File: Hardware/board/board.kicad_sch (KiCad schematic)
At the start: 0 parts

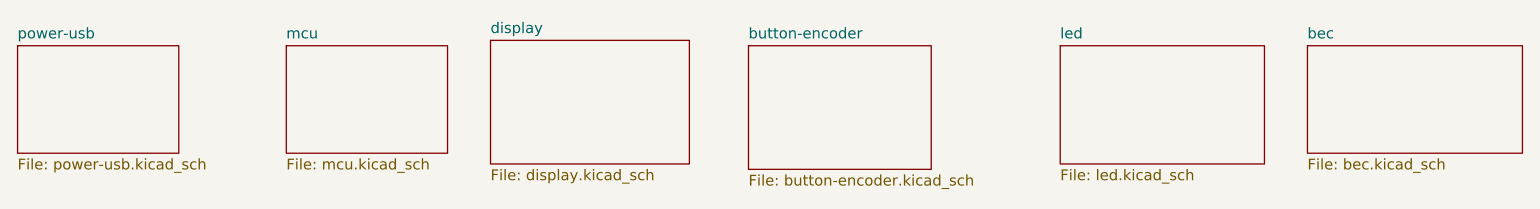
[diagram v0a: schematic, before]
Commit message: sdadsa
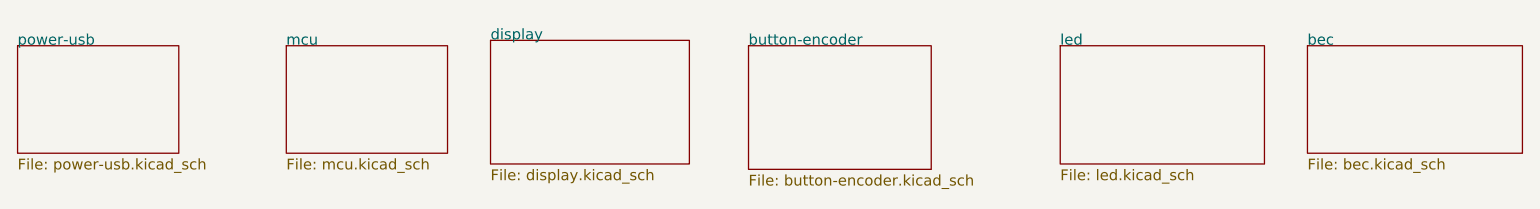
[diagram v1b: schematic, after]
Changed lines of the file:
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@@
 					(size 1.27 1.27)
 				)
-				(justify left bottom)
+				(justify left)
 			)
 		)
@@
 					(size 1.27 1.27)
 				)
-				(justify left bottom)
+				(justify left)
 			)
 		)
@@
 					(size 1.27 1.27)
 				)
-				(justify left bottom)
+				(justify left)
 			)
 		)
@@
 					(size 1.27 1.27)
 				)
-				(justify left bottom)
+				(justify left)
 			)
 		)
@@
 					(size 1.27 1.27)
 				)
-				(justify left bottom)
+				(justify left)
 			)
 		)
@@
 					(size 1.27 1.27)
 				)
-				(justify left bottom)
-			)
-		)
+				(justify left)
+			)
+		)
